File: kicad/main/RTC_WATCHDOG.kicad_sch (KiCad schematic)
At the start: 14 parts, among them U1 PCF85063AT_AY_C5151540, U12 74LVC1G07SE-7, U16 74LVC1G07SE-7, X2 ABS07-120-32_768KHZ-T

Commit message: Fix edge cut; no-CM STEP
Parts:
- C56, C57, C86: footprint Capacitor_SMD:C_0603_1608Metric_Pad1.08x0.95mm_HandSolder -> Capacitor_SMD:C_0603_1608Metric
- R102, R126, R134, R135: footprint Resistor_SMD:R_0603_1608Metric_Pad0.98x0.95mm_HandSolder -> Resistor_SMD:R_0603_1608Metric
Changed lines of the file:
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@@
 		)
 		(instances
-			(project "oomwoo-kicad"
+			(project "Main"
 				(path "/dbcfb655-8d45-4808-9a74-2a0eb03372e8/7f043eef-851b-4fc7-bc1b-c170004bfbd9"
 					(reference "#PWR0677")
@@
 		)
 		(instances
-			(project "oomwoo-kicad"
+			(project "Main"
 				(path "/dbcfb655-8d45-4808-9a74-2a0eb03372e8/7f043eef-851b-4fc7-bc1b-c170004bfbd9"
 					(reference "U12")
@@
 		)
 		(instances
-			(project "oomwoo-kicad"
+			(project "Main"
 				(path "/dbcfb655-8d45-4808-9a74-2a0eb03372e8/7f043eef-851b-4fc7-bc1b-c170004bfbd9"
 					(reference "#PWR0672")
@@
 			)
 		)
-		(property "Footprint" "Resistor_SMD:R_0603_1608Metric_Pad0.98x0.95mm_HandSolder"
+		(property "Footprint" "Resistor_SMD:R_0603_1608Metric"
 			(at 423.164 159.131 90)
 			(hide yes)
@@
 		)
 		(instances
-			(project "oomwoo-kicad"
+			(project "Main"
 				(path "/dbcfb655-8d45-4808-9a74-2a0eb03372e8/7f043eef-851b-4fc7-bc1b-c170004bfbd9"
 					(reference "R134")
@@
 		)
 		(instances
-			(project "oomwoo-kicad"
+			(project "Main"
 				(path "/dbcfb655-8d45-4808-9a74-2a0eb03372e8/7f043eef-851b-4fc7-bc1b-c170004bfbd9"
 					(reference "C52")
@@
 		)
 		(instances
-			(project "oomwoo-kicad"
+			(project "Main"
 				(path "/dbcfb655-8d45-4808-9a74-2a0eb03372e8/7f043eef-851b-4fc7-bc1b-c170004bfbd9"
 					(reference "#PWR098")
@@
 			)
 		)
-		(property "Footprint" "Resistor_SMD:R_0603_1608Metric_Pad0.98x0.95mm_HandSolder"
+		(property "Footprint" "Resistor_SMD:R_0603_1608Metric"
 			(at 359.664 148.209 90)
 			(hide yes)
@@
 		)
 		(instances
-			(project "oomwoo-kicad"
+			(project "Main"
 				(path "/dbcfb655-8d45-4808-9a74-2a0eb03372e8/7f043eef-851b-4fc7-bc1b-c170004bfbd9"
 					(reference "R126")
@@
 		)
 		(instances
-			(project "oomwoo-kicad"
+			(project "Main"
 				(path "/dbcfb655-8d45-4808-9a74-2a0eb03372e8/7f043eef-851b-4fc7-bc1b-c170004bfbd9"
 					(reference "#PWR099")
@@
 		)
 		(instances
-			(project "oomwoo-kicad"
+			(project "Main"
 				(path "/dbcfb655-8d45-4808-9a74-2a0eb03372e8/7f043eef-851b-4fc7-bc1b-c170004bfbd9"
 					(reference "X2")
@@
 		)
 		(instances
-			(project "oomwoo-kicad"
+			(project "Main"
 				(path "/dbcfb655-8d45-4808-9a74-2a0eb03372e8/7f043eef-851b-4fc7-bc1b-c170004bfbd9"
 					(reference "C53")
@@
 			)
 		)
-		(property "Footprint" "Resistor_SMD:R_0603_1608Metric_Pad0.98x0.95mm_HandSolder"
+		(property "Footprint" "Resistor_SMD:R_0603_1608Metric"
 			(at 282.829 144.399 90)
 			(hide yes)
@@
 		)
 		(instances
-			(project "oomwoo-kicad"
+			(project "Main"
 				(path "/dbcfb655-8d45-4808-9a74-2a0eb03372e8/7f043eef-851b-4fc7-bc1b-c170004bfbd9"
 					(reference "R135")
@@
 		)
 		(instances
-			(project "oomwoo-kicad"
+			(project "Main"
 				(path "/dbcfb655-8d45-4808-9a74-2a0eb03372e8/7f043eef-851b-4fc7-bc1b-c170004bfbd9"
 					(reference "#PWR0675")
@@
 		)
 		(instances
-			(project "oomwoo-kicad"
+			(project "Main"
 				(path "/dbcfb655-8d45-4808-9a74-2a0eb03372e8/7f043eef-851b-4fc7-bc1b-c170004bfbd9"
 					(reference "#PWR0674")
@@
 			)
 		)
-		(property "Footprint" "Capacitor_SMD:C_0603_1608Metric_Pad1.08x0.95mm_HandSolder"
+		(property "Footprint" "Capacitor_SMD:C_0603_1608Metric"
 			(at 406.7048 172.085 0)
 			(hide yes)
@@
 		)
 		(instances
-			(project "oomwoo-kicad"
+			(project "Main"
 				(path "/dbcfb655-8d45-4808-9a74-2a0eb03372e8/7f043eef-851b-4fc7-bc1b-c170004bfbd9"
 					(reference "C57")
@@
 		)
 		(instances
-			(project "oomwoo-kicad"
+			(project "Main"
 				(path "/dbcfb655-8d45-4808-9a74-2a0eb03372e8/7f043eef-851b-4fc7-bc1b-c170004bfbd9"
 					(reference "#PWR0676")
@@
 			)
 		)
-		(property "Footprint" "Resistor_SMD:R_0603_1608Metric_Pad0.98x0.95mm_HandSolder"
+		(property "Footprint" "Resistor_SMD:R_0603_1608Metric"
 			(at 343.154 148.209 90)
 			(hide yes)
@@
 		)
 		(instances
-			(project "oomwoo-kicad"
+			(project "Main"
 				(path "/dbcfb655-8d45-4808-9a74-2a0eb03372e8/7f043eef-851b-4fc7-bc1b-c170004bfbd9"
 					(reference "R102")
@@
 		)
 		(instances
-			(project "oomwoo-kicad"
+			(project "Main"
 				(path "/dbcfb655-8d45-4808-9a74-2a0eb03372e8/7f043eef-851b-4fc7-bc1b-c170004bfbd9"
 					(reference "U16")
@@
 		)
 		(instances
-			(project "oomwoo-kicad"
+			(project "Main"
 				(path "/dbcfb655-8d45-4808-9a74-2a0eb03372e8/7f043eef-851b-4fc7-bc1b-c170004bfbd9"
 					(reference "#PWR0673")
@@
 			)
 		)
-		(property "Footprint" "Capacitor_SMD:C_0603_1608Metric_Pad1.08x0.95mm_HandSolder"
+		(property "Footprint" "Capacitor_SMD:C_0603_1608Metric"
 			(at 355.6 156.5402 0)
 			(hide yes)
@@
 		)
 		(instances
-			(project "oomwoo-kicad"
+			(project "Main"
 				(path "/dbcfb655-8d45-4808-9a74-2a0eb03372e8/7f043eef-851b-4fc7-bc1b-c170004bfbd9"
 					(reference "C86")
@@
 			)
 		)
-		(property "Footprint" "Capacitor_SMD:C_0603_1608Metric_Pad1.08x0.95mm_HandSolder"
+		(property "Footprint" "Capacitor_SMD:C_0603_1608Metric"
 			(at 184.4548 170.18 0)
 			(hide yes)
@@
 		)
 		(instances
-			(project "oomwoo-kicad"
+			(project "Main"
 				(path "/dbcfb655-8d45-4808-9a74-2a0eb03372e8/7f043eef-851b-4fc7-bc1b-c170004bfbd9"
 					(reference "C56")
@@
 		)
 		(instances
-			(project "oomwoo-kicad"
+			(project "Main"
 				(path "/dbcfb655-8d45-4808-9a74-2a0eb03372e8/7f043eef-851b-4fc7-bc1b-c170004bfbd9"
 					(reference "#PWR0671")
@@
 		)
 		(instances
-			(project "oomwoo-kicad"
+			(project "Main"
 				(path "/dbcfb655-8d45-4808-9a74-2a0eb03372e8/7f043eef-851b-4fc7-bc1b-c170004bfbd9"
 					(reference "#PWR068")
@@
 		)
 		(instances
-			(project "oomwoo-kicad"
+			(project "Main"
 				(path "/dbcfb655-8d45-4808-9a74-2a0eb03372e8/7f043eef-851b-4fc7-bc1b-c170004bfbd9"
 					(reference "C87")
@@
 		)
 		(instances
-			(project "oomwoo-kicad"
+			(project "Main"
 				(path "/dbcfb655-8d45-4808-9a74-2a0eb03372e8/7f043eef-851b-4fc7-bc1b-c170004bfbd9"
 					(reference "U1")

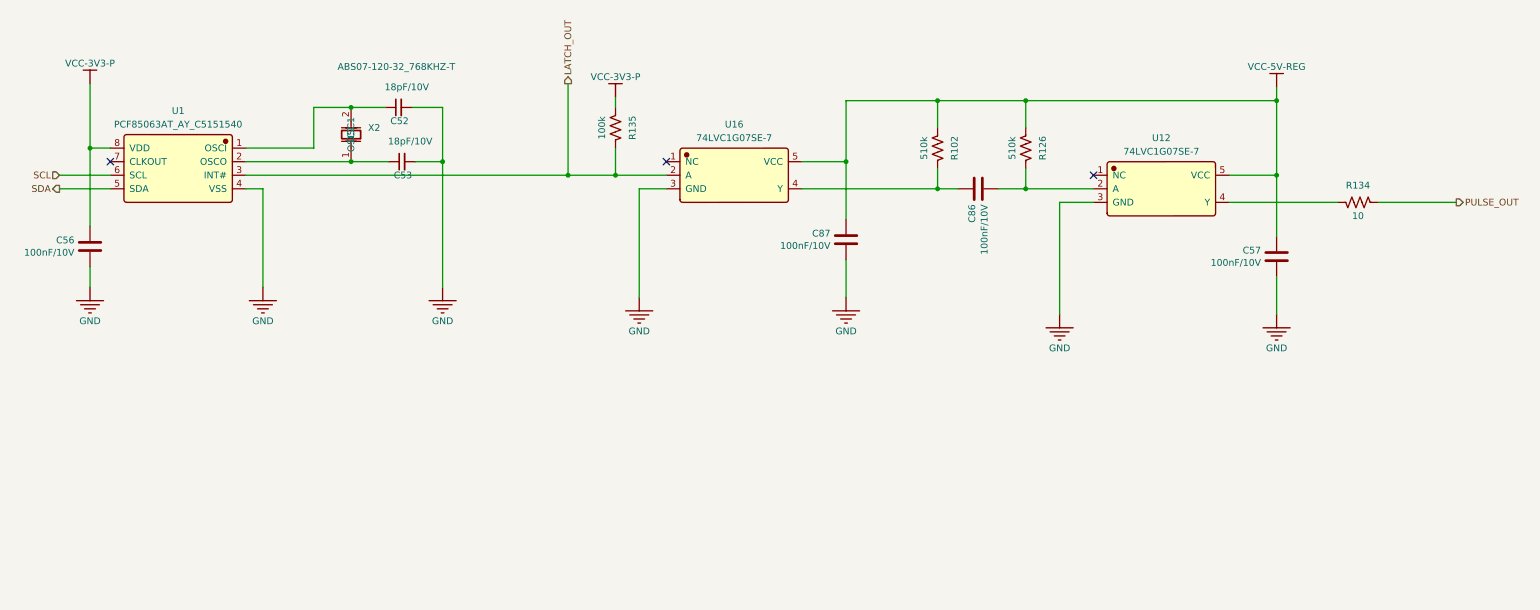
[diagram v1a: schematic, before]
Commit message: Schematic fixes, 1st round of review
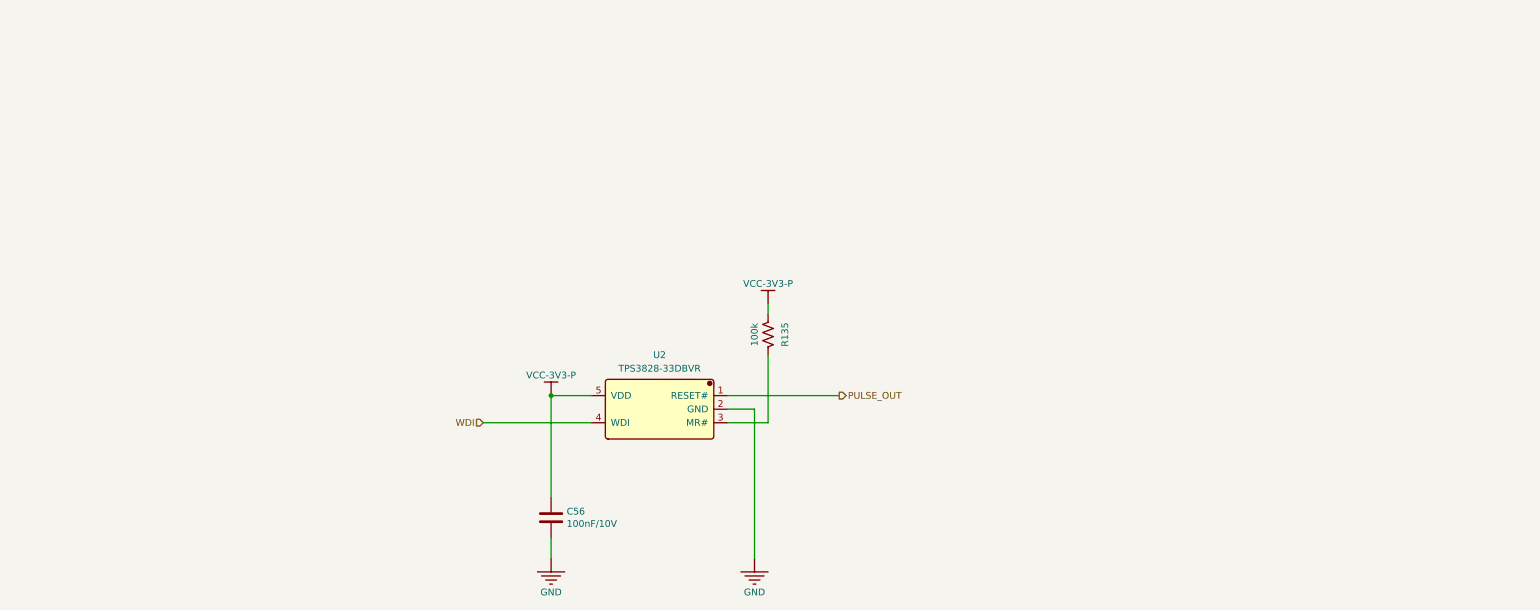
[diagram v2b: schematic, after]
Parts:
- removed C52, C53: 18pF/10V, Capacitor_SMD:C_0603_1608Metric, symbol Device:C_Small
- removed C57, C86: 100nF/10V, Capacitor_SMD:C_0603_1608Metric, symbol Device:C
- removed C87: 100nF/10V, Capacitor_SMD:C_0603_1608Metric_Pad1.08x0.95mm_HandSolder, symbol Device:C
- removed R102, R126: 510k, Resistor_SMD:R_0603_1608Metric, symbol Device:R_US
- removed R134: 10, Resistor_SMD:R_0603_1608Metric, symbol Device:R_US
- removed U1: PCF85063AT_AY_C5151540, JLCImport:PCF85063AT_AY_C5151540, symbol JLCImport:PCF85063AT_AY_C5151540
- removed U12, U16: 74LVC1G07SE-7, JLCImport:74LVC1G07SE-7, symbol JLCImport:74LVC1G07SE-7
- removed X2: ABS07-120-32_768KHZ-T, JLCImport:ABS07-120-32_768KHZ-T, symbol JLCImport:ABS07-120-32_768KHZ-T
- added U2: TPS3828-33DBVR, JLCImport:TPS3828-33DBVR, symbol JLCImport:TPS3828-33DBVR
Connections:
- net GND: now also U2.2 (GND)
- net PULSE_OUT: now also U2.1 (RESET#)
- net VCC-3V3-P: now also U2.5 (VDD)
- net LATCH_OUT: no longer names the net of R135.2
- net LATCH_OUT: now also U2.3 (MR#)
- new net WDI: U2.4 (WDI)
- no-connect marks 3 -> 0
